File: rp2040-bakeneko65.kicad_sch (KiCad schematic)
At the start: 1 part

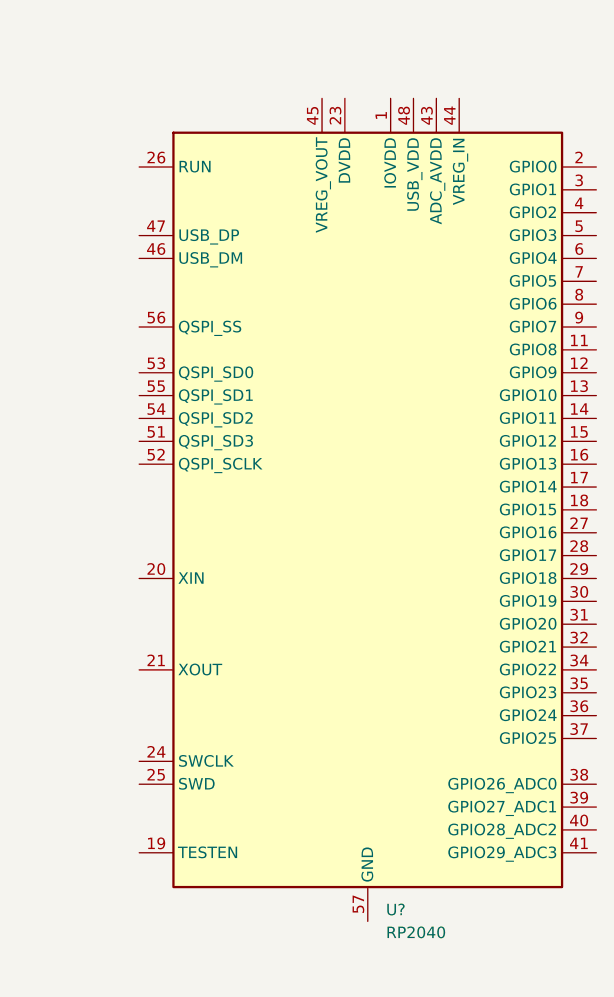
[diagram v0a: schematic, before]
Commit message: Some schematic work
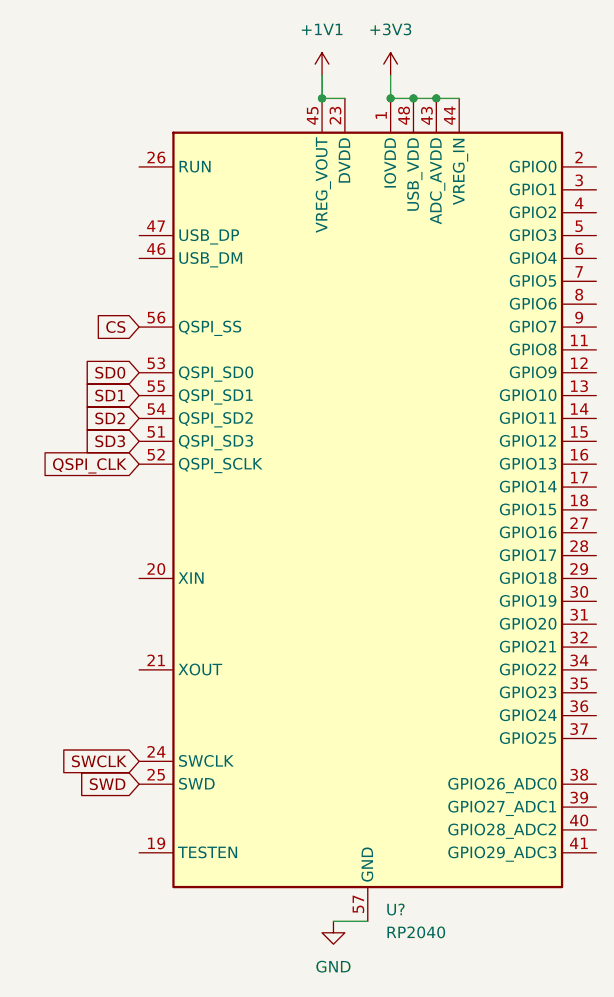
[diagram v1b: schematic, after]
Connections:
- net +3V3: now reaches U?.1 (IOVDD), U?.10 (IOVDD), U?.22 (IOVDD), U?.33 (IOVDD), U?.42 (IOVDD), U?.49 (IOVDD)
- net +3V3: now also U?.43 (ADC_AVDD), U?.44 (VREG_IN), U?.48 (USB_VDD)
- net +1V1: now reaches U?.23 (DVDD), U?.50 (DVDD)
- net +1V1: now also U?.45 (VREG_VOUT)
- net SWCLK: now reaches U?.24 (SWCLK)
- net SWD: now reaches U?.25 (SWD)
- net SD3: now reaches U?.51 (QSPI_SD3)
- net QSPI_CLK: now reaches U?.52 (QSPI_SCLK)
- net SD0: now reaches U?.53 (QSPI_SD0)
- net SD2: now reaches U?.54 (QSPI_SD2)
- net SD1: now reaches U?.55 (QSPI_SD1)
- net CS: now reaches U?.56 (QSPI_SS)
- net GND: now reaches U?.57 (GND)
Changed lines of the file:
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@@
 (kicad_sch (version 20211123) (generator eeschema)
   (paper "A4")
+  (junction (at 81.28 29.21) (diameter 0) (color 0 0 0 0)
+  )
+  (junction (at 78.74 29.21) (diameter 0) (color 0 0 0 0)
+  )
+  (junction (at 76.2 29.21) (diameter 0) (color 0 0 0 0)
+  )
+  (junction (at 68.58 29.21) (diameter 0) (color 0 0 0 0)
+  )
+  (wire (pts (xy 76.2 29.21) (xy 78.74 29.21))
+    (stroke (width 0) (type default) (color 0 0 0 0))
+  )
+  (wire (pts (xy 76.2 26.67) (xy 76.2 29.21))
+    (stroke (width 0) (type default) (color 0 0 0 0))
+  )
+  (wire (pts (xy 69.85 120.65) (xy 73.66 120.65))
+    (stroke (width 0) (type default) (color 0 0 0 0))
+  )
+  (wire (pts (xy 78.74 29.21) (xy 81.28 29.21))
+    (stroke (width 0) (type default) (color 0 0 0 0))
+  )
+  (wire (pts (xy 68.58 29.21) (xy 71.12 29.21))
+    (stroke (width 0) (type default) (color 0 0 0 0))
+  )
+  (wire (pts (xy 81.28 29.21) (xy 83.82 29.21))
+    (stroke (width 0) (type default) (color 0 0 0 0))
+  )
+  (wire (pts (xy 68.58 26.67) (xy 68.58 29.21))
+    (stroke (width 0) (type default) (color 0 0 0 0))
+  )
+  (global_label "CS" (shape input) (at 48.26 54.61 180) (fields_autoplaced)
+    (effects (font (size 1.27 1.27)) (justify right))
+    (property "Intersheet References" "${INTERSHEET_REFS}" (id 0) (at 43.3674 54.5306 0)
+      (effects (font (size 1.27 1.27)) (justify right) hide)
+    )
+  )
+  (global_label "QSPI_CLK" (shape input) (at 48.26 69.85 180) (fields_autoplaced)
+    (effects (font (size 1.27 1.27)) (justify right))
+    (property "Intersheet References" "${INTERSHEET_REFS}" (id 0) (at 36.8964 69.7706 0)
+      (effects (font (size 1.27 1.27)) (justify right) hide)
+    )
+  )
+  (global_label "SWCLK" (shape input) (at 48.26 102.87 180) (fields_autoplaced)
+    (effects (font (size 1.27 1.27)) (justify right))
+    (property "Intersheet References" "${INTERSHEET_REFS}" (id 0) (at 39.6179 102.7906 0)
+      (effects (font (size 1.27 1.27)) (justify right) hide)
+    )
+  )
+  (global_label "SWD" (shape input) (at 48.26 105.41 180) (fields_autoplaced)
+    (effects (font (size 1.27 1.27)) (justify right))
+    (property "Intersheet References" "${INTERSHEET_REFS}" (id 0) (at 41.9159 105.3306 0)
+      (effects (font (size 1.27 1.27)) (justify right) hide)
+    )
+  )
+  (global_label "SD1" (shape input) (at 48.26 62.23 180) (fields_autoplaced)
+    (effects (font (size 1.27 1.27)) (justify right))
+    (property "Intersheet References" "${INTERSHEET_REFS}" (id 0) (at 42.1579 62.1506 0)
+      (effects (font (size 1.27 1.27)) (justify right) hide)
+    )
+  )
+  (global_label "SD2" (shape input) (at 48.26 64.77 180) (fields_autoplaced)
+    (effects (font (size 1.27 1.27)) (justify right))
+    (property "Intersheet References" "${INTERSHEET_REFS}" (id 0) (at 42.1579 64.6906 0)
+      (effects (font (size 1.27 1.27)) (justify right) hide)
+    )
+  )
+  (global_label "SD0" (shape input) (at 48.26 59.69 180) (fields_autoplaced)
+    (effects (font (size 1.27 1.27)) (justify right))
+    (property "Intersheet References" "${INTERSHEET_REFS}" (id 0) (at 42.1579 59.6106 0)
+      (effects (font (size 1.27 1.27)) (justify right) hide)
+    )
+  )
+  (global_label "SD3" (shape input) (at 48.26 67.31 180) (fields_autoplaced)
+    (effects (font (size 1.27 1.27)) (justify right))
+    (property "Intersheet References" "${INTERSHEET_REFS}" (id 0) (at 42.1579 67.2306 0)
+      (effects (font (size 1.27 1.27)) (justify right) hide)
+    )
+  )
+  (symbol (lib_id "power:GND") (at 69.85 120.65 0) (unit 1)
+    (in_bom yes) (on_board yes) (fields_autoplaced)
+    (property "Reference" "#PWR?" (id 0) (at 69.85 127 0)
+      (effects (font (size 1.27 1.27)) hide)
+    )
+    (property "Value" "GND" (id 1) (at 69.85 125.73 0))
+    (property "Footprint" "" (id 2) (at 69.85 120.65 0)
+      (effects (font (size 1.27 1.27)) hide)
+    )
+    (property "Datasheet" "" (id 3) (at 69.85 120.65 0)
+      (effects (font (size 1.27 1.27)) hide)
+    )
+    (pin "1")
+  )
+  (symbol (lib_id "power:+3V3") (at 76.2 26.67 0) (unit 1)
+    (in_bom yes) (on_board yes) (fields_autoplaced)
+    (property "Reference" "#PWR?" (id 0) (at 76.2 30.48 0)
+      (effects (font (size 1.27 1.27)) hide)
+    )
+    (property "Value" "+3V3" (id 1) (at 76.2 21.59 0))
+    (property "Footprint" "" (id 2) (at 76.2 26.67 0)
+      (effects (font (size 1.27 1.27)) hide)
+    )
+    (property "Datasheet" "" (id 3) (at 76.2 26.67 0)
+      (effects (font (size 1.27 1.27)) hide)
+    )
+    (pin "1")
+  )
   (symbol (lib_id "MCU_RaspberryPi:RP2040") (at 73.66 74.93 0) (unit 1)
     (in_bom yes) (on_board yes) (fields_autoplaced)
@@
     (pin "9")
   )
+  (symbol (lib_id "power:+1V1") (at 68.58 26.67 0) (unit 1)
+    (in_bom yes) (on_board yes) (fields_autoplaced)
+    (property "Reference" "#PWR?" (id 0) (at 68.58 30.48 0)
+      (effects (font (size 1.27 1.27)) hide)
+    )
+    (property "Value" "+1V1" (id 1) (at 68.58 21.59 0))
+    (property "Footprint" "" (id 2) (at 68.58 26.67 0)
+      (effects (font (size 1.27 1.27)) hide)
+    )
+    (property "Datasheet" "" (id 3) (at 68.58 26.67 0)
+      (effects (font (size 1.27 1.27)) hide)
+    )
+    (pin "1")
+  )
   (sheet_instances
     (path "/" (page "1"))
   )
   (symbol_instances
+    (path "/0429f72c-16b0-4744-90f4-bc022597ca0f"
+      (reference "#PWR?") (unit 1) (value "GND") (footprint "")
+    )
+    (path "/10a7cbd1-d76a-46cc-8e26-d9c6917c2458"
+      (reference "#PWR?") (unit 1) (value "+3V3") (footprint "")
+    )
+    (path "/7e675cbf-1df0-4184-8643-46226909b2bc"
+      (reference "#PWR?") (unit 1) (value "+1V1") (footprint "")
+    )
     (path "/7983fcb6-a16e-4782-bd80-c146df78a95c"
       (reference "U?") (unit 1) (value "RP2040") (footprint "Package_DFN_QFN:QFN-56-1EP_7x7mm_P0.4mm_EP3.2x3.2mm")
